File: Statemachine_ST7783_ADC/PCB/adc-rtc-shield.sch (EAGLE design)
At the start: 12 parts, among them IC1 RV-3029-C2, IC3 AT24C32

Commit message: -remove documentation, -add shield pcb
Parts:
- removed BATT1: 2032, El_Mech:CR2032_HOLDSMD
- removed C103: 100nF, rcl:C-EUC0603
- removed IC1: RV-3029-C2, crystal:RV-3029-C2
- removed IC3: AT24C32, PKJ:24C32
- removed JP1: (no value), pinhead:PINHD-1X5/90
- removed R1: 2K2, rcl:R-EU_R0603
- removed R90: 330R, rcl:R-EU_R0603
- added BATT2: 2032, El_Mech:CR2032_HOLDSMD
- added C10, C11, C12, C13, C19, C2, C20, C21, C22, C23, C24, C25, C26, C5, C8, C9: 10n, Passiv:C_KER
- added C16, C3, C6: 100n, Passiv:C_KER
- added C27: 100nF, rcl:C-EUC0402S
- added IC2: RV_3049_C2, RTC_Quarz:RV_3049_C2
- added J10, J11, J12, J13, J14, J15, J16, J9: MC1,5/2-G-3,5, PHOENIX:MC1,5/2-G-3,5
- added R10, R13, R14, R15, R16, R17, R6, R7, R8, R9: 2K, Passiv:R@2
- added R11, R12, R18, R19, R20, R21, R3: 10K, Passiv:R@2
- added R22: 330R, rcl:R-EU_R0603
- added R4: 1K21, Passiv:R@2
- added R5: 909R, Passiv:R@2
- added U$1: TLC2543, HL_IC1:TLC2543
- R2: value 2K2 -> 10K; device rcl:R-EU_R0603 -> Passiv:R@2; TK 100 -> (none); TOL 1% -> (none); VOLT 50V -> (none)
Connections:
- net N$29 renamed IO1
- net N$30 renamed IO0
- removed net N$12: IC1.VBACKUP, R90.2
- removed net RESET: AD.5, POWER.3
- new net /CS-WDI: U$1./CS
- new net 3,3V: C27.1, IC2.VCC
- new net AREF: IOH.8, R10.2, R13.2, R14.2, R15.2, R16.2, R17.2, R6.1, R7.1, R8.2, R9.2
- new net CLK: U$1.CLK
- new net DATIN: U$1.DATIN
- new net DATOUT: U$1.DATOUT
- new net N$10: C3.2, R5.1, R6.2, U$1.REF-
- new net N$11: C6.2, R4.1, R7.2, U$1.REF+
- new net N$16: C2.2, R11.2, U$1.AIN1
- new net N$17: C8.2, R2.2, U$1.AIN2
- new net N$18: C9.2, R3.2, U$1.AIN3
- new net N$19: C5.2, R12.2, U$1.AIN0
- new net N$20: C23.2, R18.2, U$1.AIN4
- new net N$21: C24.2, R19.2, U$1.AIN5
- new net N$22: C25.2, R20.2, U$1.AIN6
- new net N$23: C26.2, R21.2, U$1.AIN7
- new net N$25: IC2.VBAT, R22.2
- new net N$26: IC2.CS
- new net N$27: BATT2.+, R22.1
- new net N$3: POWER.3
- new net SCK: IOH.6
- new net SPCK: IC2.SCL
- new net VCC: C16.2
- new net X1_RX4-: C13.2, J9.1.1, R12.1, R9.1
- new net X2_TX4-: C12.2, J10.1.1, R11.1, R13.1
- new net X3_RX3-: C10.2, J11.1.1, R10.1, R2.1
- new net X4_TX3-: C11.2, J12.1.1, R3.1, R8.1
- new net X5_RX2-: C19.2, J13.1.1, R14.1, R18.1
- new net X6_TX2-: C21.2, J14.1.1, R15.1, R19.1
- new net X7_RX1-: C20.2, J15.1.1, R16.1, R20.1
- new net X8_TX1-: C22.2, J16.1.1, R17.1, R21.1
- net +3V3: no longer C103.1, IC1.VDD, IC3.VCC, JP1.2, R1.2, R2.2
- net +5V: no longer JP1.1
- net AD4/SDA: now also AD.5; no longer IC1.SDA, IC3.SDA, JP1.4, R2.1
- net AD5/SCL: now also AD.6; no longer IC1.SCL, IC3.SCL, JP1.3, R1.1
- net GND: now also BATT2.-, C10.1, C11.1, C12.1, C13.1, C16.1, C19.1, C2.1, C20.1, C21.1, C22.1, C23.1, C24.1, C25.1, C26.1, C27.2, C3.1, C5.1, C6.1, C8.1, C9.1, IC2.GND, J10.2.1, J11.2.1, J12.2.1, J13.2.1, J14.2.1, J15.2.1, J16.2.1, J9.2.1, R4.2, R5.2, U$1.GND; no longer BATT1.-, C103.2, IC1.VSS, IC3.A0, IC3.A1, IC3.A2, IC3.GND, IC3.WP, JP1.5
- net MISO: now also IC2.SDO
- net MOSI: now also IC2.SDI
- net N$1: now also U$1.VCC; no longer BATT1.+, R90.1
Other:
- note added: "ADC RTC Shield"
- note removed: "TFT RESET, Pin nicht mit Arduino Borad verbinden!"
- moved on the sheet: AD, IOH, IOL, POWER

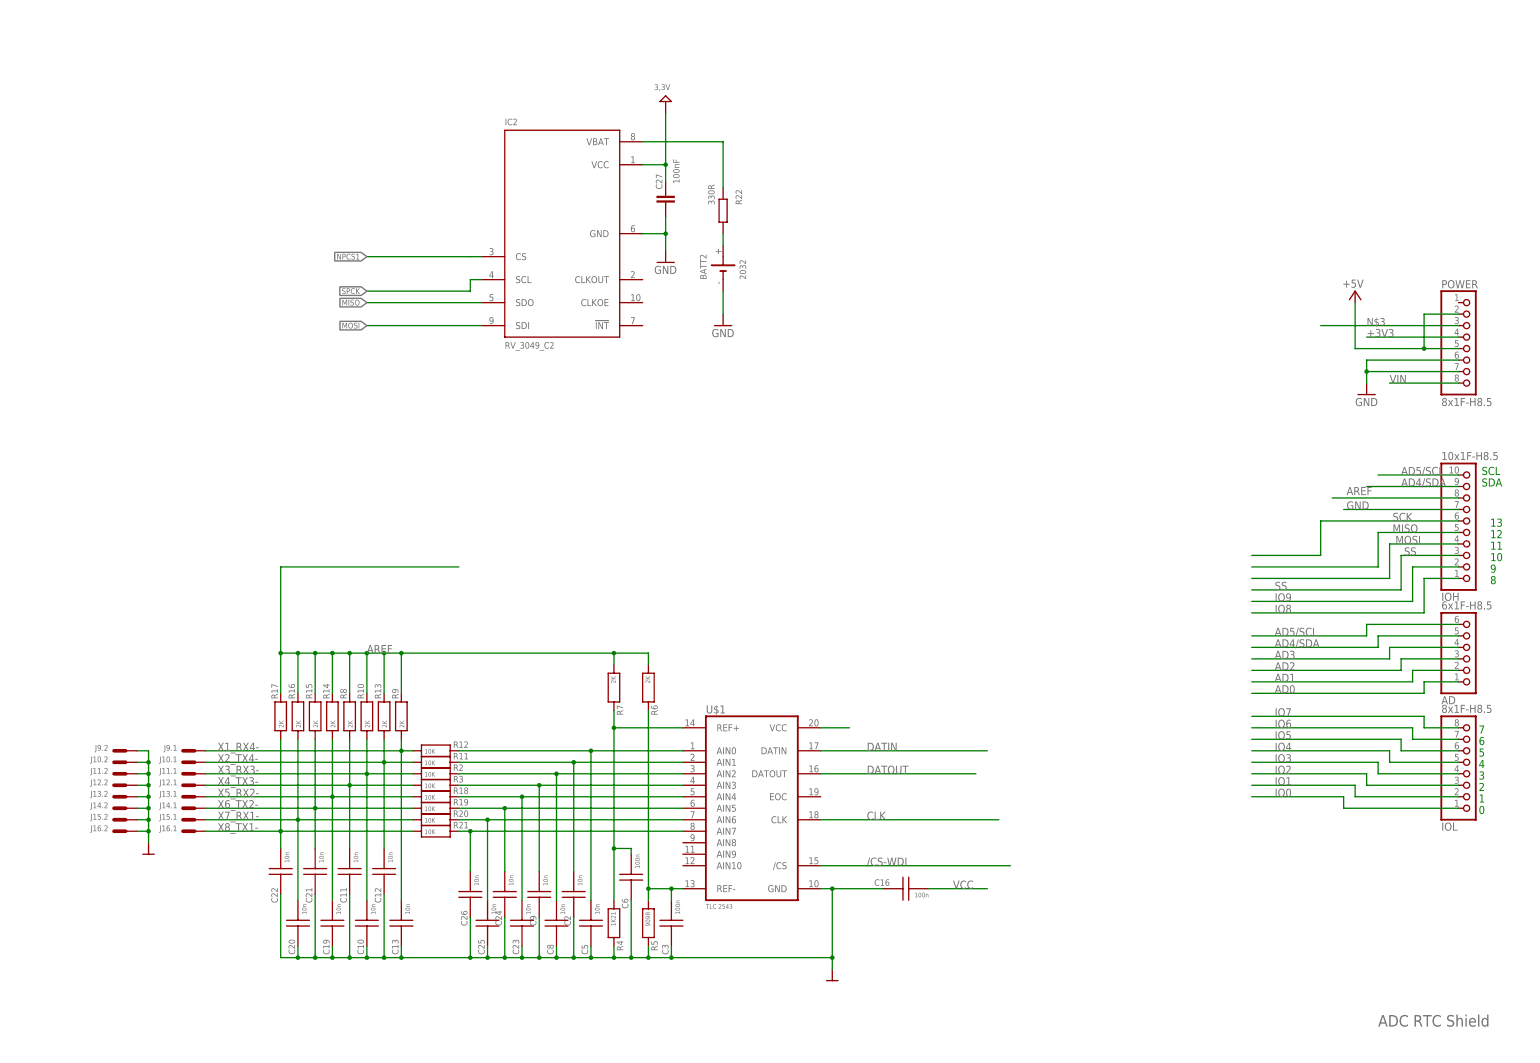
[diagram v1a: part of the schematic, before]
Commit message: cleanup
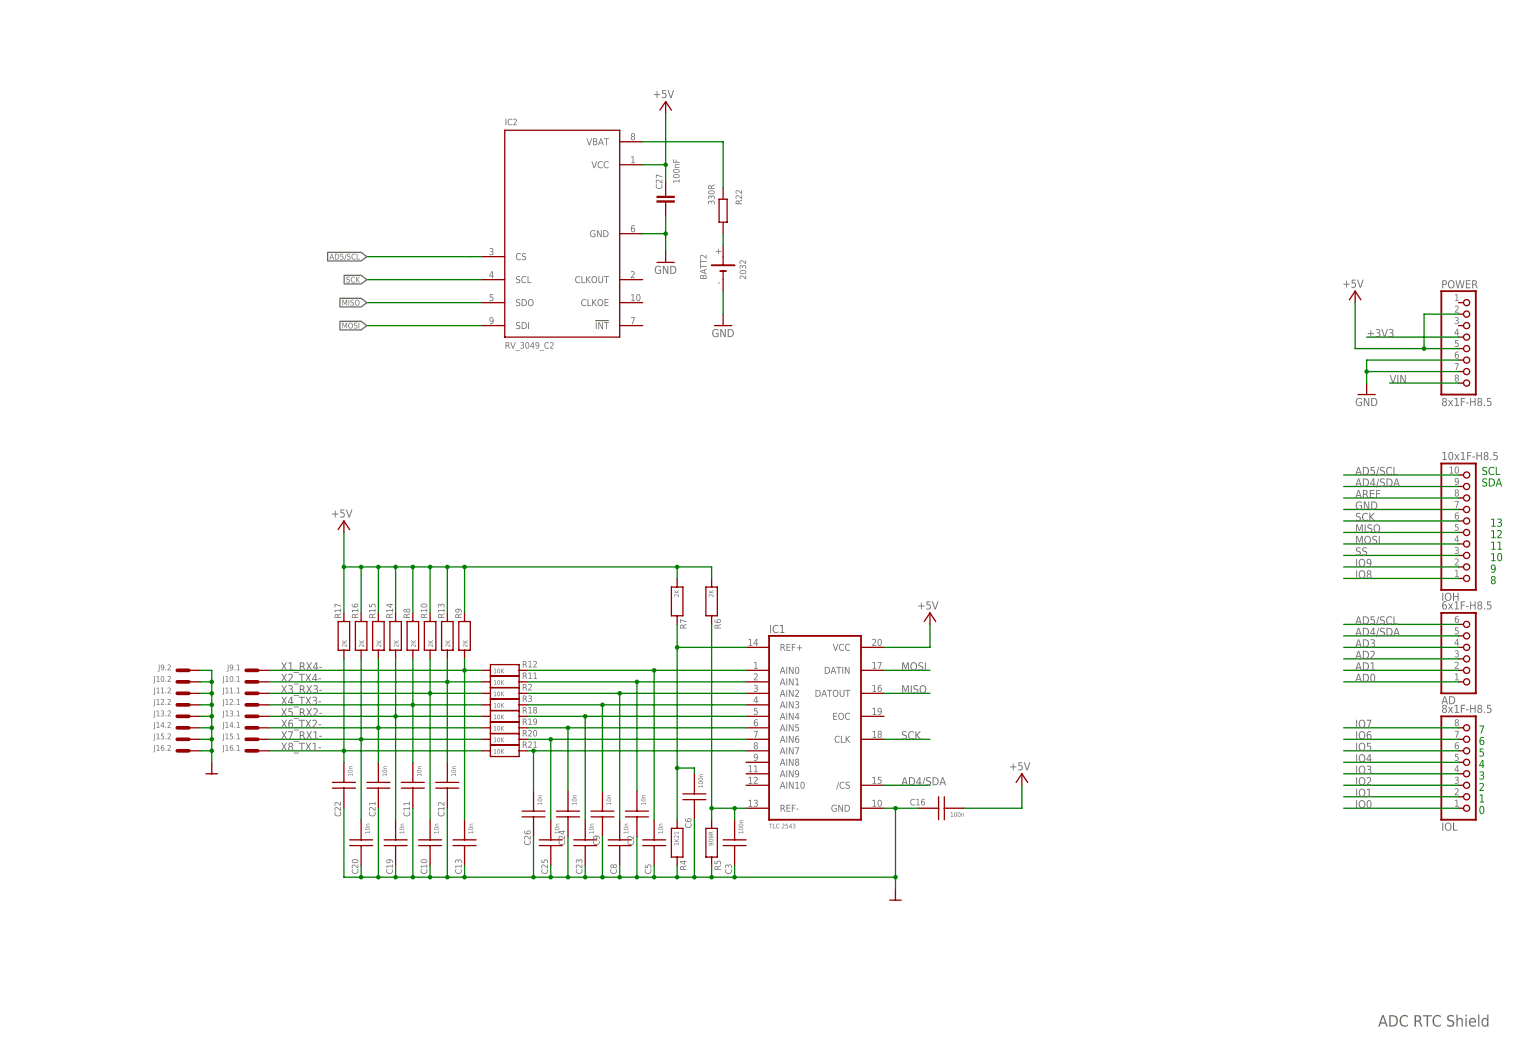
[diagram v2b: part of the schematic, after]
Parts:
- removed U$1: TLC2543, HL_IC1:TLC2543
- added IC1: TLC2543, HL_IC1:TLC2543
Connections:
- removed net /CS-WDI: U$1./CS
- removed net 3,3V: C27.1, IC2.VCC
- removed net CLK: U$1.CLK
- removed net DATIN: U$1.DATIN
- removed net DATOUT: U$1.DATOUT
- removed net N$1: U$1.VCC
- removed net N$3: POWER.3
- removed net SPCK: IC2.SCL
- removed net VCC: C16.2
- net +5V: now also C16.2, C27.1, IC1.VCC, IC2.VCC, R10.2, R13.2, R14.2, R15.2, R16.2, R17.2, R6.1, R7.1, R8.2, R9.2
- net AD4/SDA: now also IC1./CS
- net AREF: no longer R10.2, R13.2, R14.2, R15.2, R16.2, R17.2, R6.1, R7.1, R8.2, R9.2
- net GND: now also IC1.GND; no longer U$1.GND
- net MISO: now also IC1.DATOUT
- net MOSI: now also IC1.DATIN
- net N$10: now also IC1.REF-; no longer U$1.REF-
- net N$11: now also IC1.REF+; no longer U$1.REF+
- net N$16: now also IC1.AIN1; no longer U$1.AIN1
- net N$17: now also IC1.AIN2; no longer U$1.AIN2
- net N$18: now also IC1.AIN3; no longer U$1.AIN3
- net N$19: now also IC1.AIN0; no longer U$1.AIN0
- net N$20: now also IC1.AIN4; no longer U$1.AIN4
- net N$21: now also IC1.AIN5; no longer U$1.AIN5
- net N$22: now also IC1.AIN6; no longer U$1.AIN6
- net N$23: now also IC1.AIN7; no longer U$1.AIN7
- net SCK: now also IC1.CLK, IC2.SCL
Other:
- moved on the sheet: C10, C11, C12, C13, C16, C19, C2, C20, C21, C22, C23, C24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
